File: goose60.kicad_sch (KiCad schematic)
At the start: 1 part

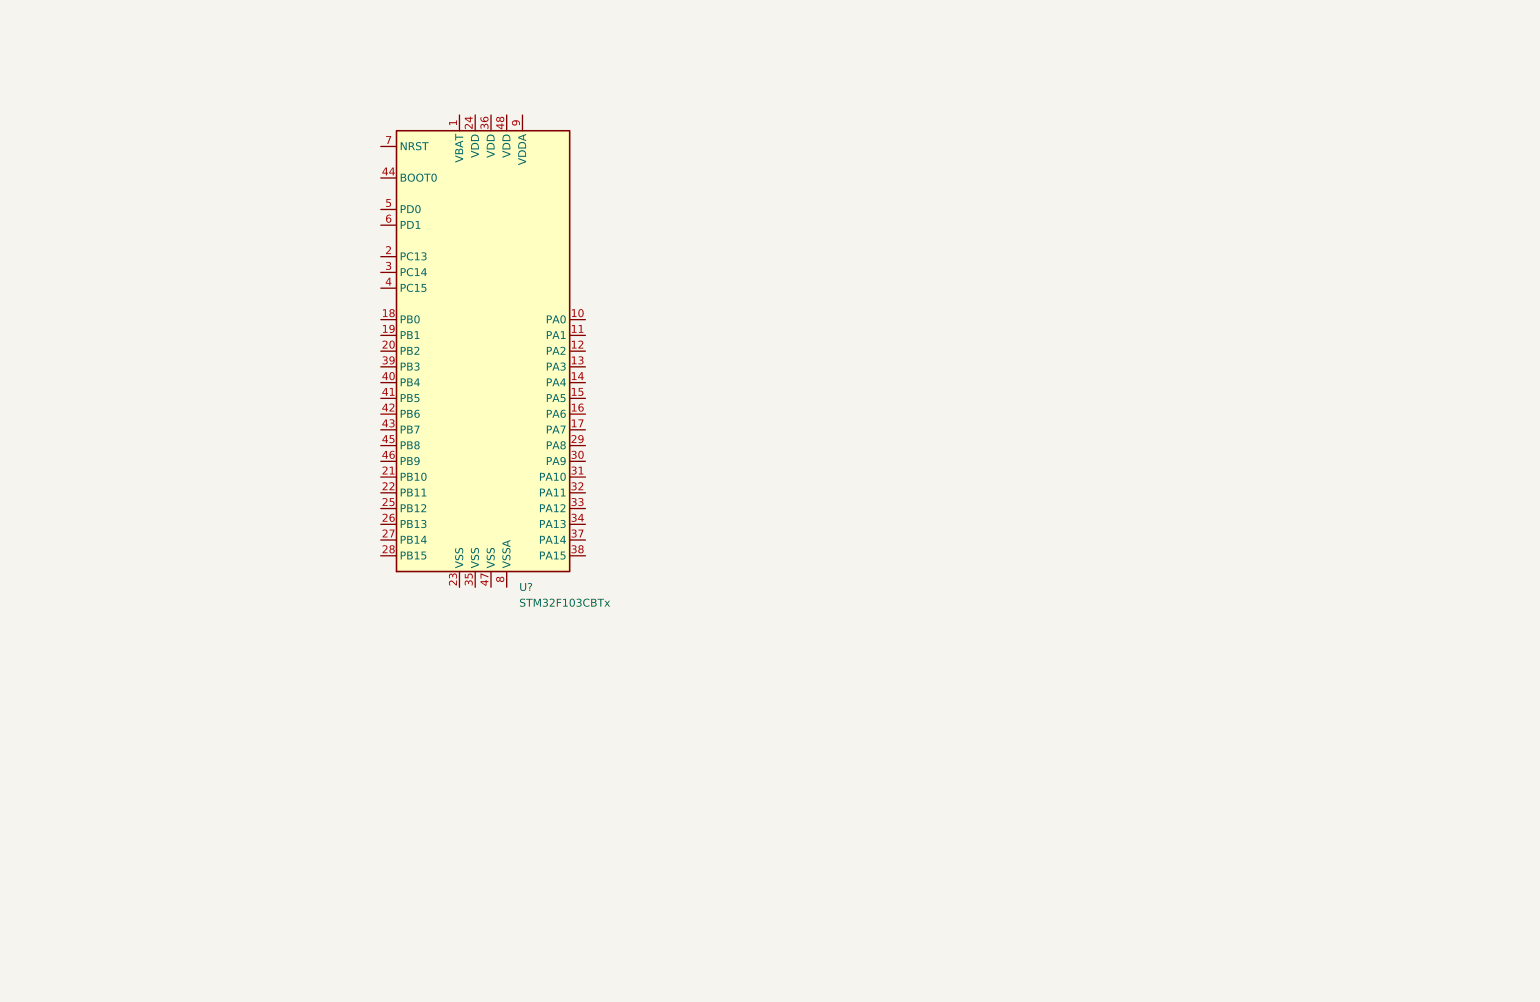
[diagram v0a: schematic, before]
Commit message: add new design
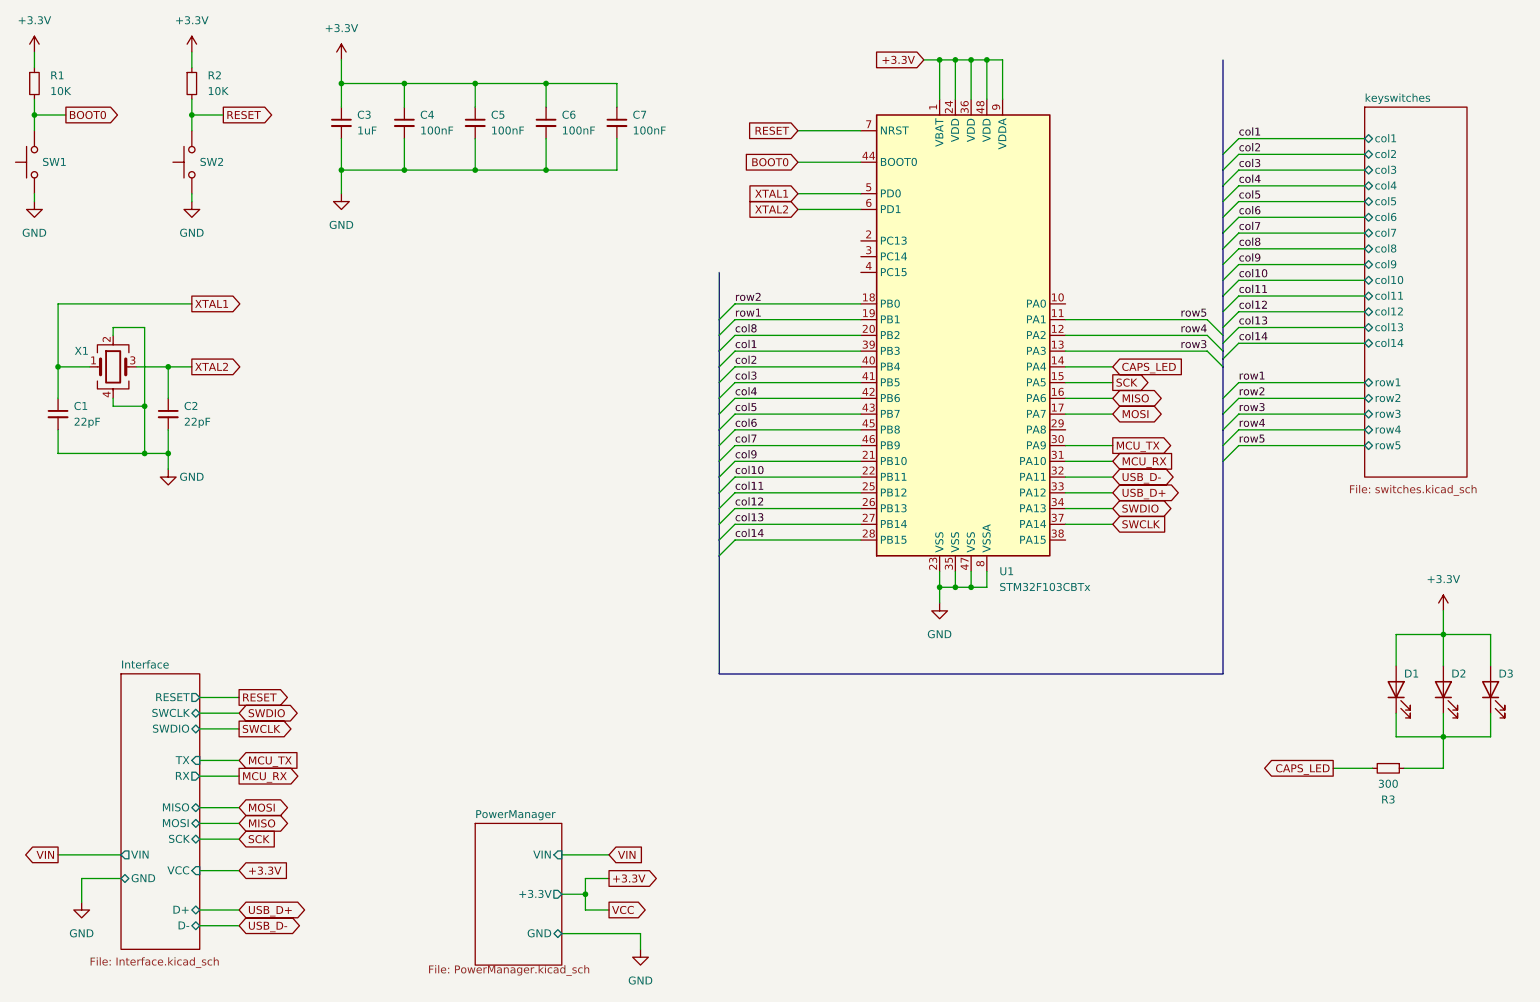
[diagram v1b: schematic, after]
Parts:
- added C1, C2: 22pF, symbol Device:C_Small
- added C3: 1uF, symbol Device:C_Small
- added C4, C5, C6, C7: 100nF, symbol Device:C_Small
- added D1, D2, D3: LED, symbol Device:LED
- added R1, R2: 10K, Resistor_SMD:R_0805_2012Metric, symbol Device:R_Small
- added R3: 300, symbol Device:R_Small
- added SW1, SW2: SW_Push, Button_Switch_SMD:SW_Push_1P1T_NO_CK_KSC6xxJ, symbol Switch:SW_Push
- added X1: Crystal_GND24, symbol Device:Crystal_GND24
- gave numbers to parts that had none: 1
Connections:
- net +3.3V: now reaches U1.1 (VBAT)
- net +3.3V: now also U1.24 (VDD), U1.36 (VDD), U1.48 (VDD), U1.9 (VDDA), C3.1, C4.1, C5.1, C6.1, C7.1, D1.2 (A), D2.2 (A), D3.2 (A), R1.1, R2.1
- net row5: now reaches U1.11 (PA1)
- net row4: now reaches U1.12 (PA2)
- net row3: now reaches U1.13 (PA3)
- net CAPS_LED: now reaches U1.14 (PA4)
- net CAPS_LED: now also R3.2
- net SCK: now reaches U1.15 (PA5)
- net MISO: now reaches U1.16 (PA6)
- net MOSI: now reaches U1.17 (PA7)
- net row2: now reaches U1.18 (PB0)
- net row1: now reaches U1.19 (PB1)
- net col8: now reaches U1.20 (PB2)
- net col9: now reaches U1.21 (PB10)
- net col10: now reaches U1.22 (PB11)
- net GND: now reaches U1.23 (VSS)
- net GND: now also U1.35 (VSS), U1.47 (VSS), U1.8 (VSSA), C1.2, C2.2, C3.2, C4.2, C5.2, C6.2, C7.2, SW1.1, SW2.1, X1.2, X1.4
- net col11: now reaches U1.25 (PB12)
- net col12: now reaches U1.26 (PB13)
- net col13: now reaches U1.27 (PB14)
- net col14: now reaches U1.28 (PB15)
- net MCU_TX: now reaches U1.30 (PA9)
- net MCU_RX: now reaches U1.31 (PA10)
- net USB_D-: now reaches U1.32 (PA11)
- net USB_D+: now reaches U1.33 (PA12)
- net SWDIO: now reaches U1.34 (PA13)
- net SWCLK: now reaches U1.37 (PA14)
- net col1: now reaches U1.39 (PB3)
- net col2: now reaches U1.40 (PB4)
- net col3: now reaches U1.41 (PB5)
- net col4: now reaches U1.42 (PB6)
- net col5: now reaches U1.43 (PB7)
- net BOOT0: now reaches U1.44 (BOOT0)
- net BOOT0: now also R1.2, SW1.2
- net col6: now reaches U1.45 (PB8)
- net col7: now reaches U1.46 (PB9)
- net XTAL1: now reaches U1.5 (PD0)
- net XTAL1: now also C1.1, X1.1
- net XTAL2: now reaches U1.6 (PD1)
- net XTAL2: now also C2.1, X1.3
- net RESET: now reaches U1.7 (NRST)
- net RESET: now also R2.2, SW2.2
- new net: D1.1 (K), D2.1 (K), D3.1 (K), R3.1
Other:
- added sheet Interface (Interface.kicad_sch)
- added sheet PowerManager (PowerManager.kicad_sch)
- added sheet keyswitches (switches.kicad_sch)
- moved on the sheet: U1
